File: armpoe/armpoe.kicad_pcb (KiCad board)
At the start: 2 copper layers, 60 x 60 mm, 107 parts, among them J101 RJ45, Q101 Si4848DY, Q102 Si4848DY, Q103 Si4848DY, Q104 Si2325DS, T101 H2019, T102 HA3691-AL, U101 PM8803, U102 OPTO-TRANSISTOR, U103 TS431, U201 STM32F107XXX-LQFP64, U202 KSZ8001S, U203 MCP1603, X202 CRYSTAL

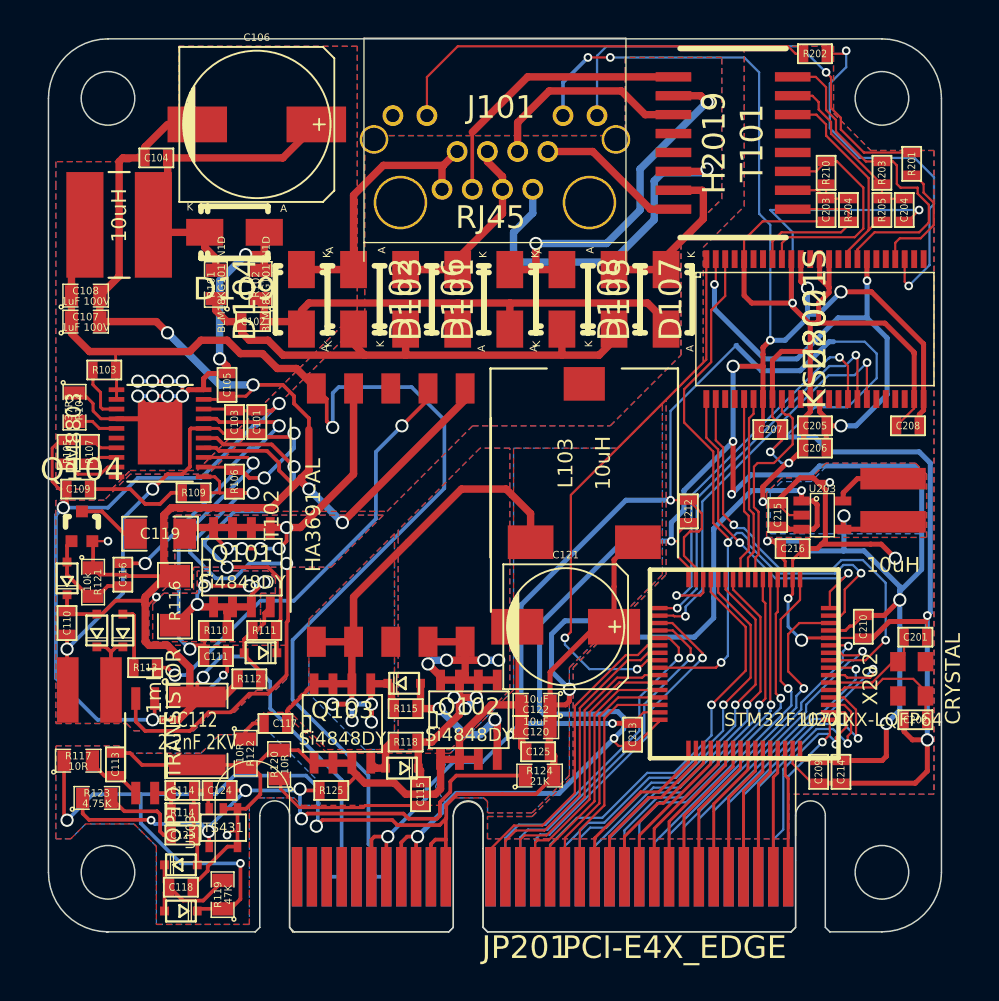
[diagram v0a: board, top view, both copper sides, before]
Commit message: All routed. Again.
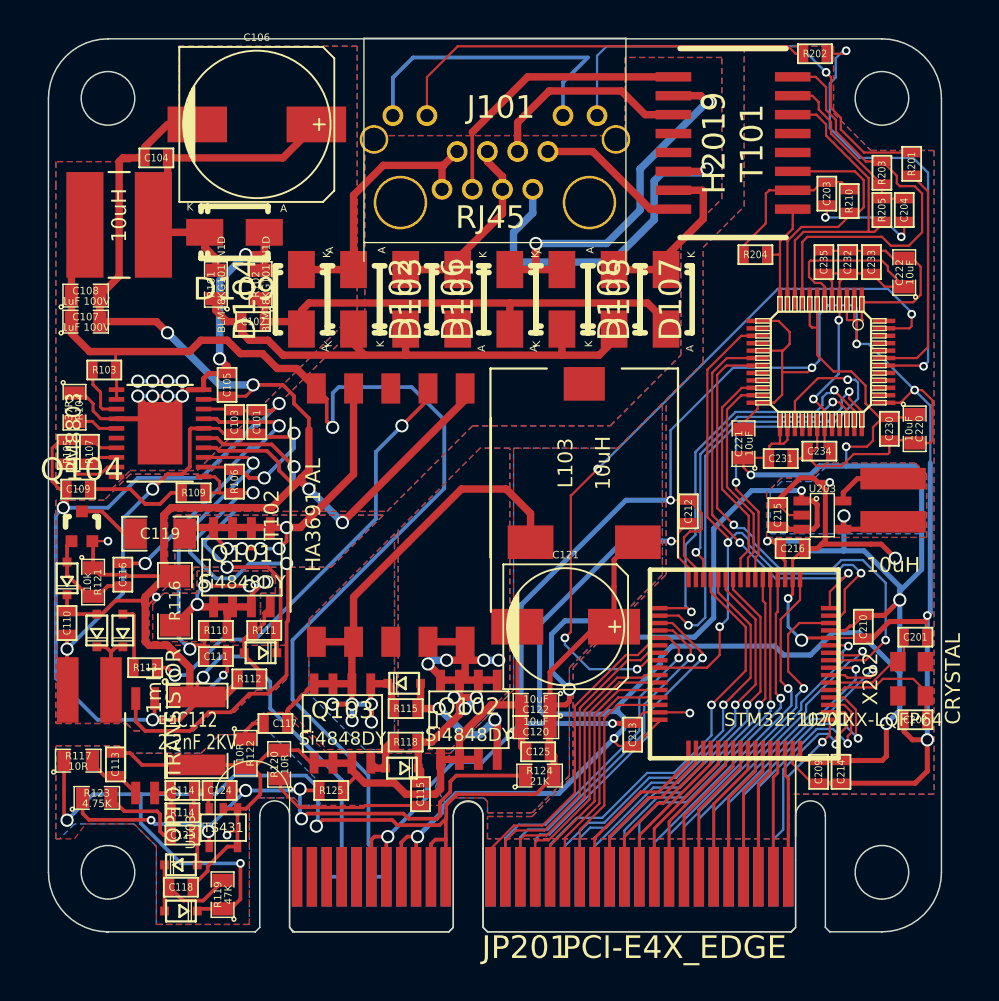
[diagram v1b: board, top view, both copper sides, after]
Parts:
- removed C205, C208: 1uF, SM0603
- removed C206, C207: 100nF, SM0603
- added C220: 10uF, SM0805, F.Cu at (238.2, 86.2)
- added C221: 10uF, SM0805, F.Cu at (226.7, 87.2)
- added C222: 10uF, SM0805, F.Cu at (237.5, 75.7)
- added C230: 100nF, SM0603, F.Cu at (236.5, 86.2)
- added C231: 100nF, SM0603, F.Cu at (229.2, 88.2)
- added C232: 100nF, SM0603, F.Cu at (233.7, 75.0)
- added C233: 100nF, SM0603, F.Cu at (235.3, 75.0)
- added C234: 100nF, SM0603, F.Cu at (231.8, 87.7)
- added C235: 100nF, SM0603, F.Cu at (232.1, 75.0)
- U202: value KSZ8001S -> KSZ8041; footprint SSOP48 -> -TQFP48
- moved R204 6.93 mm to (227.5, 74.5), turned to 0 degrees
- moved R210 2.45 mm to (233.8, 70.9), turned to 270 degrees
- moved U202 2.24 mm to (231.9, 81.7), turned to 180 degrees
- moved C203 1.10 mm to (232.3, 70.4)
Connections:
- R201 pad 1: N-0000072 -> N-0000063
- R202 pad 1: N-0000073 -> N-0000062
- U202 pad 1: /MCU/RMII_MDIO -> GND
- U202 pad 10: (no net) -> /MCU/RX+
- U202 pad 11: (no net) -> /MCU/TX-
- U202 pad 12: GND -> /MCU/TX+
- U202 pad 13: +1.8V -> GND
- U202 pad 15: (no net) -> /MCU/MCO_25
- U202 pad 16: /MCU/RMII_TXEN -> (no net)
- U202 pad 17: /MCU/RMII_TX0 -> GND
- U202 pad 18: /MCU/RMII_TX1 -> /MCU/RMII_MDIO
- U202 pad 19: (no net) -> /MCU/RMII_MDC
- U202 pad 2: /MCU/RMII_MDC -> GND
- U202 pad 22: (no net) -> /MCU/RMII_RX1
- U202 pad 23: GND -> /MCU/RMII_RX0
- U202 pad 24: +3.3V -> GND
- U202 pad 25: (no net) -> +3.3V
- U202 pad 26: (no net) -> +3.3V
- U202 pad 27: N-0000073 -> /MCU/RMII_CRX_DV
- U202 pad 28: N-0000072 -> (no net)
- U202 pad 3: (no net) -> GND
- U202 pad 30: (no net) -> GND
- U202 pad 32: /MCU/RX- -> (no net)
- U202 pad 33: /MCU/RX+ -> (no net)
- U202 pad 34: (no net) -> /MCU/RMII_TXEN
- U202 pad 35: GND -> /MCU/RMII_TX0
- U202 pad 36: GND -> /MCU/RMII_TX1
- U202 pad 37: (no net) -> GND
- U202 pad 38: +3.3V -> (no net)
- U202 pad 39: GND -> (no net)
- U202 pad 4: (no net) -> +1.8V
- U202 pad 40: /MCU/TX- -> (no net)
- U202 pad 41: /MCU/TX+ -> (no net)
- U202 pad 42: (no net) -> N-0000062
- U202 pad 43: (no net) -> N-0000063
- U202 pad 44: GND -> (no net)
- U202 pad 46: /MCU/MCO_25 -> (no net)
- U202 pad 47: +1.8V -> /MCU/ETH_RST
- U202 pad 48: /MCU/ETH_RST -> (no net)
- U202 pad 5: /MCU/RMII_RX1 -> +1.8V
- U202 pad 6: /MCU/RMII_RX0 -> +1.8V
- U202 pad 8: GND -> +3.3V
- U202 pad 9: /MCU/RMII_CRX_DV -> /MCU/RX-
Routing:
- net N-0000062: track 0.00 -> 30.8 mm, vias 0 -> 2
- net GND: track 314.8 -> 289.3 mm, vias 16 -> 17
- net N-0000073: track 25.4 -> 0.00 mm, vias 2 -> 0
- net +3.3V: track 191.4 -> 173.8 mm, vias 13 -> 9
- net N-0000063: track 0.00 -> 15.4 mm
- net /MCU/RMII_CRX_DV: track 14.4 -> 27.4 mm, vias 0 -> 2
- net /MCU/ETH_RST: track 37.1 -> 49.6 mm, vias 2 -> 4
- net N-0000072: track 8.06 -> 0.00 mm
- net /MCU/RX+: track 13.9 -> 21.5 mm
- net /MCU/RX-: track 22.4 -> 28.8 mm
- net /MCU/TXCT: track 4.95 -> 10.8 mm
- net /MCU/RMII_TXEN: track 27.0 -> 21.2 mm
- net /MCU/3.3V: track 15.1 -> 20.8 mm, vias 2 -> 0
- net /MCU/MCO_25: track 49.2 -> 43.9 mm
- net /MCU/RMII_MDIO: track 21.9 -> 26.9 mm
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
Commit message: This is what was sent off, I belive. I'm in the process fo fixing the errors now
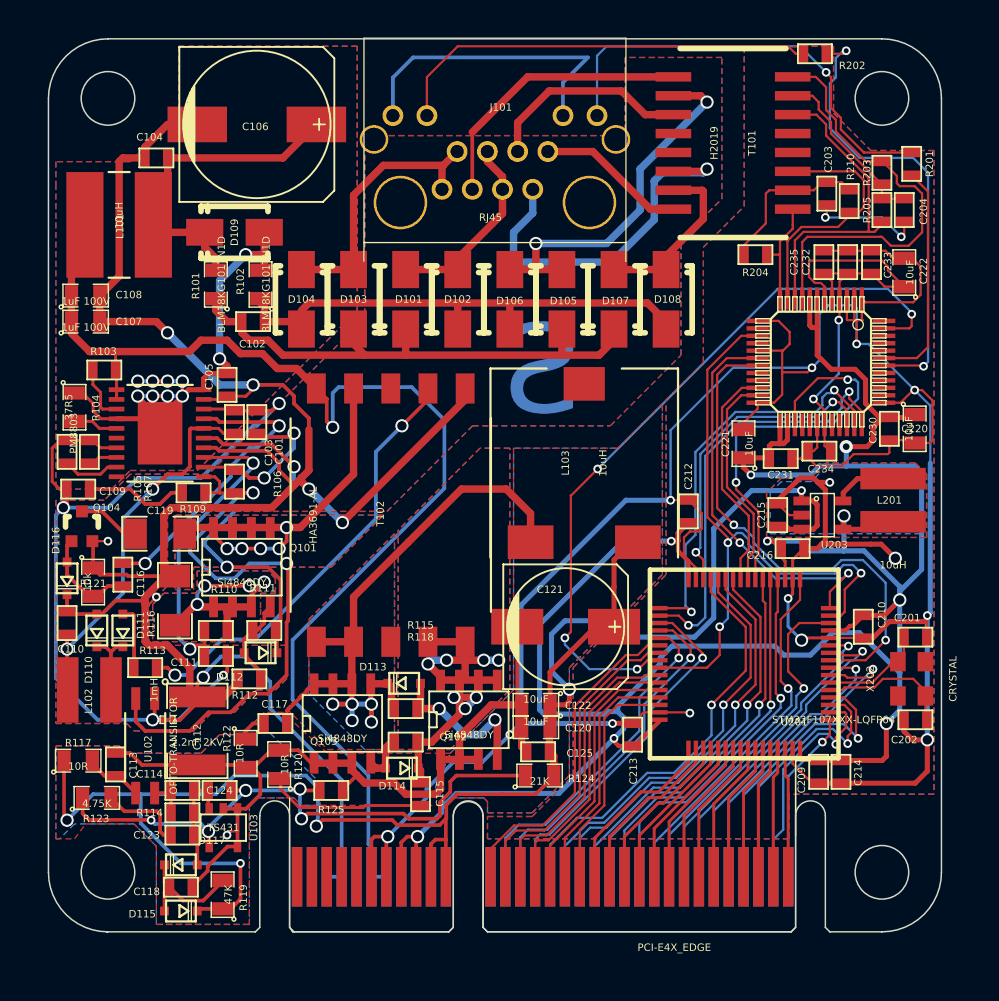
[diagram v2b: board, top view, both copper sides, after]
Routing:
- net /ARTN: track 60.9 -> 61.6 mm
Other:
- board text added: "G"
- board text added: "S"
- board text added: "STM32F107 PoE Board"
- board text added: "Scott Gilliland"
- board text added: "smg.ideacraft.org"
